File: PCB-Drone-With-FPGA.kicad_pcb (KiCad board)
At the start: 4 copper layers, 100 x 100 mm, 45 parts, among them J501 SMA-RP, U1 10CL040_F484, U401 ICM-20948, U402 BNO055, U403 DPS422XTSA1, U404 MCP3208, U405 TXB0104PWR, U501 nRF24L01P, U502 RFX2401C, X501 16MHz

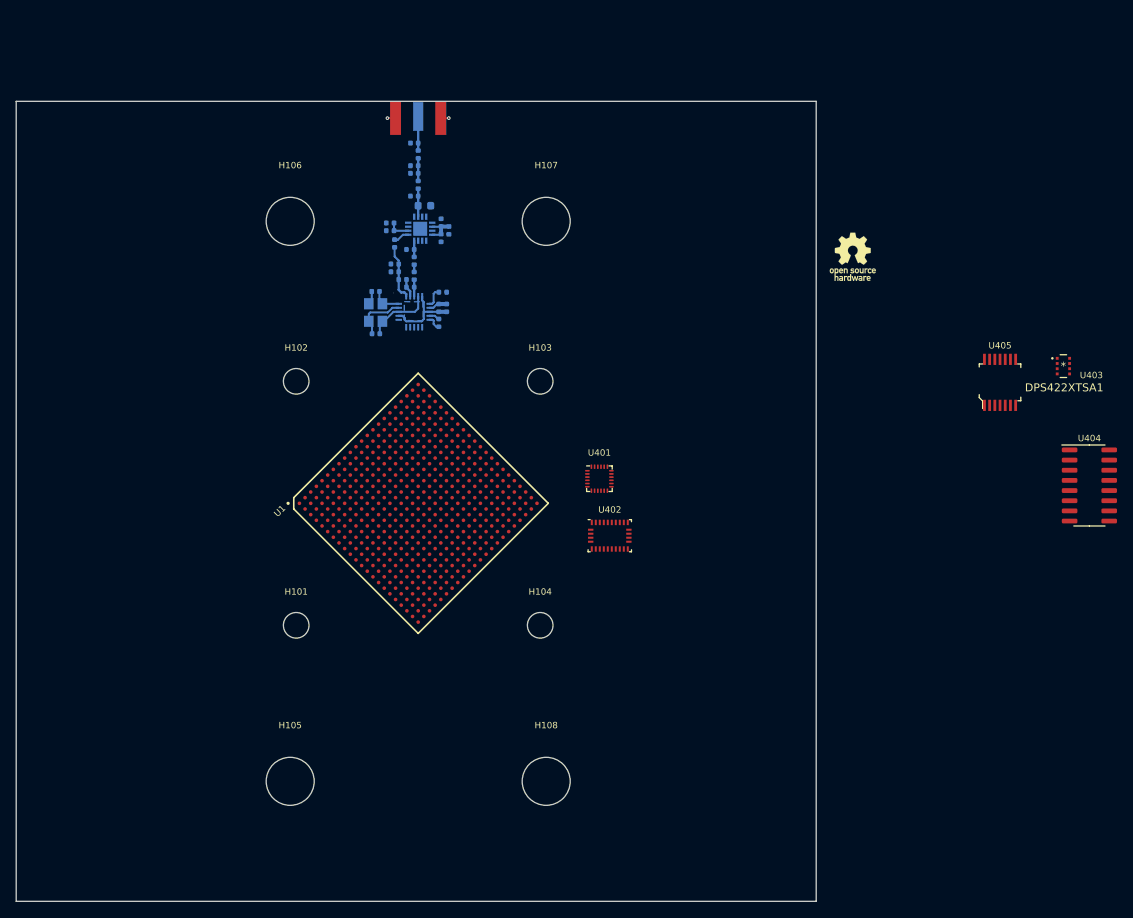
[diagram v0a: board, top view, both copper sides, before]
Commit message: More of the same
Signed-off-by: Eldalote <Eldalote.Electronics@gmail.com>
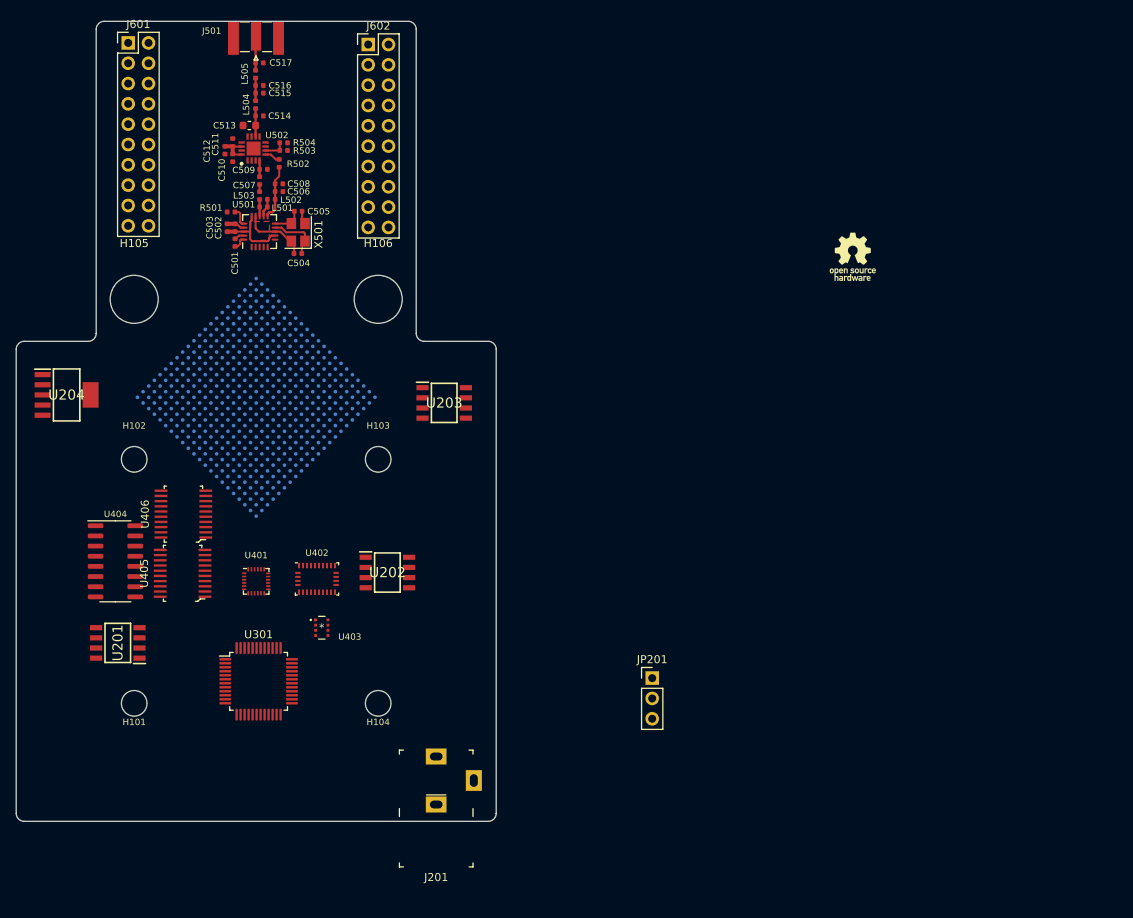
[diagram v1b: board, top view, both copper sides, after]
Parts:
- removed H107, H108: MountingHole, MountingHole:MountingHole_6mm
- added J201: PJ-102A, digikey-footprints:Barrel_Jack_5.5mmODx2.1mmID_PJ-102A, F.Cu at (152.5, 134.9)
- added J601: Conn_02x10_Row_Letter_First, Connector_PinHeader_2.54mm:PinHeader_2x10_P2.54mm_Vertical, F.Cu at (114.0, 42.7)
- added J602: Conn_02x10_Row_Letter_First, Connector_PinHeader_2.54mm:PinHeader_2x10_P2.54mm_Vertical, F.Cu at (144.0, 42.9)
- added JP201: Jumper_NC_Dual, Connector_PinHeader_2.54mm:PinHeader_1x03_P2.54mm_Vertical, F.Cu at (179.5, 122.1)
- added U201: TPS54331DR, SamacSys_Parts:SOIC127P600X175-8N, F.Cu at (112.7, 117.7)
- added U202: TPS54331DR, SamacSys_Parts:SOIC127P600X175-8N, F.Cu at (146.4, 108.9)
- added U203: TPS54331DR, SamacSys_Parts:SOIC127P600X175-8N, F.Cu at (153.5, 87.7)
- added U204: TPS73701DCQ, SamacSys_Parts:SOT127P706X180-6N, F.Cu at (106.3, 86.7)
- added U301: FT232H, Package_QFP:LQFP-48_7x7mm_P0.5mm, F.Cu at (130.3, 122.5)
- added U406: TXB0108PWR, digikey-footprints:TSSOP-20_W4.4mm, F.Cu at (120.9, 101.6)
- C501, C502, C503, C504, C505, C506, C507, C508, C509, C510, C511, C512, C513, C514, C515, C516, C517, J501, L501, L502, L503, L504, L505, R501, R502, R503, R504, U501, U502, X501: moved to F.Cu
- U1: moved to B.Cu
- U405: value TXB0104PWR -> TXB0108PWR; footprint digikey-footprints:TSSOP-14_W4.4mm -> digikey-footprints:TSSOP-20_W4.4mm
- moved U404 122.1 mm to (112.4, 107.5)
- moved U405 104.9 mm to (120.8, 109.0), turned to 90 degrees
- moved U403 98.3 mm to (138.2, 115.8)
- moved H105 63.3 mm to (114.8, 74.8)
- moved U401 44.8 mm to (130.0, 110.0)
- moved U402 37.0 mm to (137.6, 109.7)
- moved C512 29.7 mm to (126.1, 56.1)
- moved C503 29.2 mm to (126.4, 65.8)
- moved R501 28.3 mm to (126.9, 63.8), turned to 180 degrees
- moved C511 27.9 mm to (127.1, 55.1)
- moved C510 27.9 mm to (127.1, 57.1)
- moved C502 27.4 mm to (127.4, 65.8)
- moved C501 27.4 mm to (127.4, 67.7)
- moved U1 24.2 mm to (130.0, 87.0), turned to 315 degrees
- moved C513 24.1 mm to (129.1, 53.0), turned to 0 degrees
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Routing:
- net GND: track 18.1 -> 14.1 mm, vias 2 -> 0
- added copper zone on F.Cu, net GND
- removed copper zone on B.Cu, net GND
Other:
- board size 100 x 100 mm -> 60 x 100 mm
